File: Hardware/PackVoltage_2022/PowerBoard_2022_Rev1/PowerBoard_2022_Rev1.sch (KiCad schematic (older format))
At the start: 0 parts

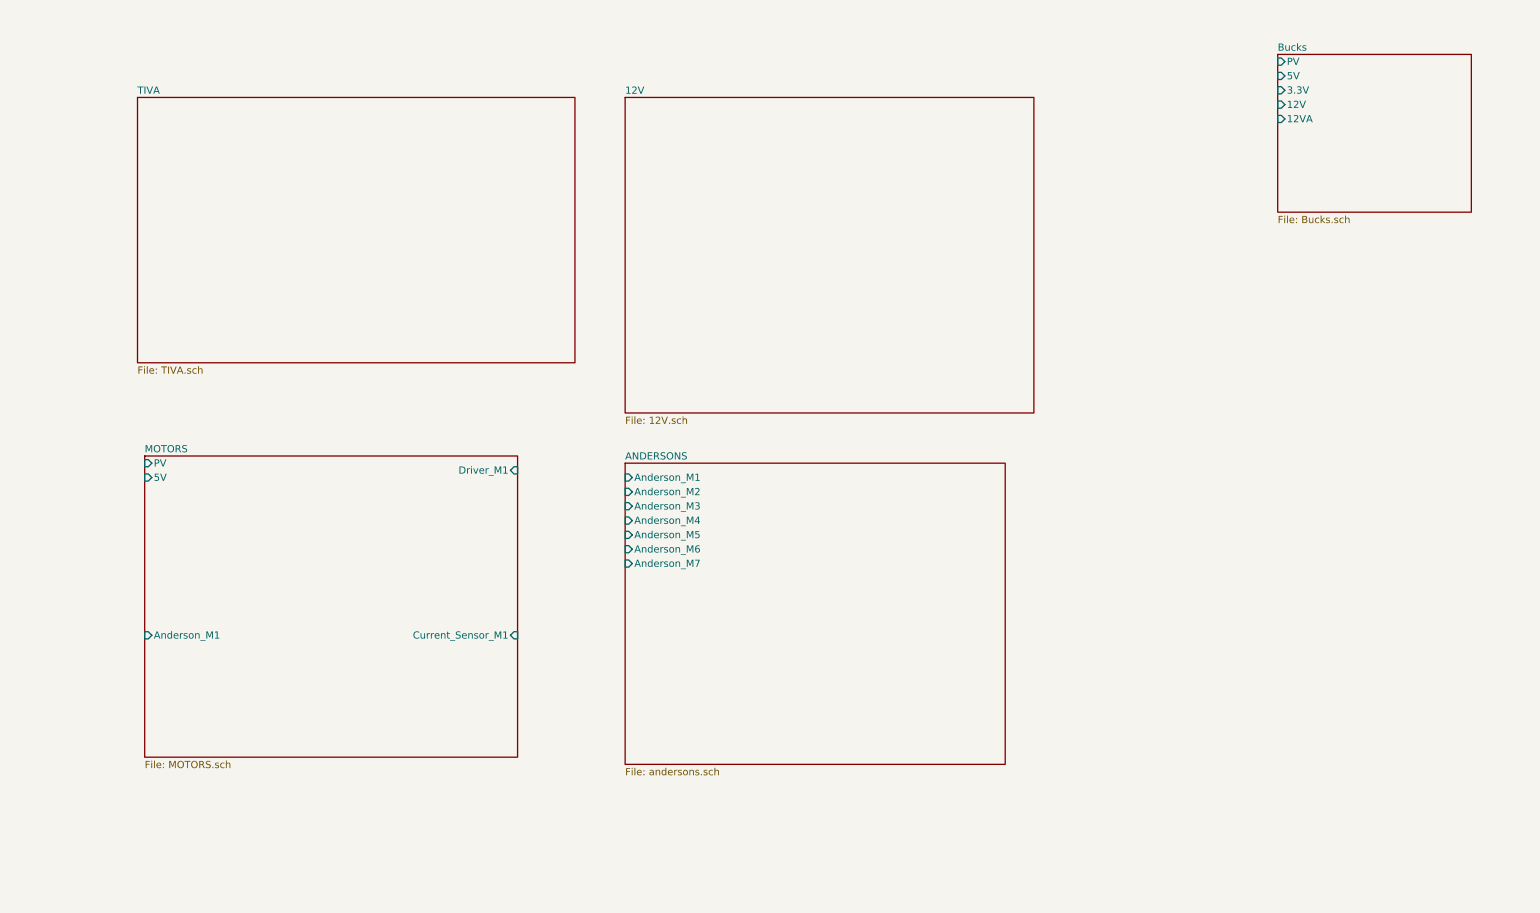
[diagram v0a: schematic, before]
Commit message: 12V stuff and hierarchical tags
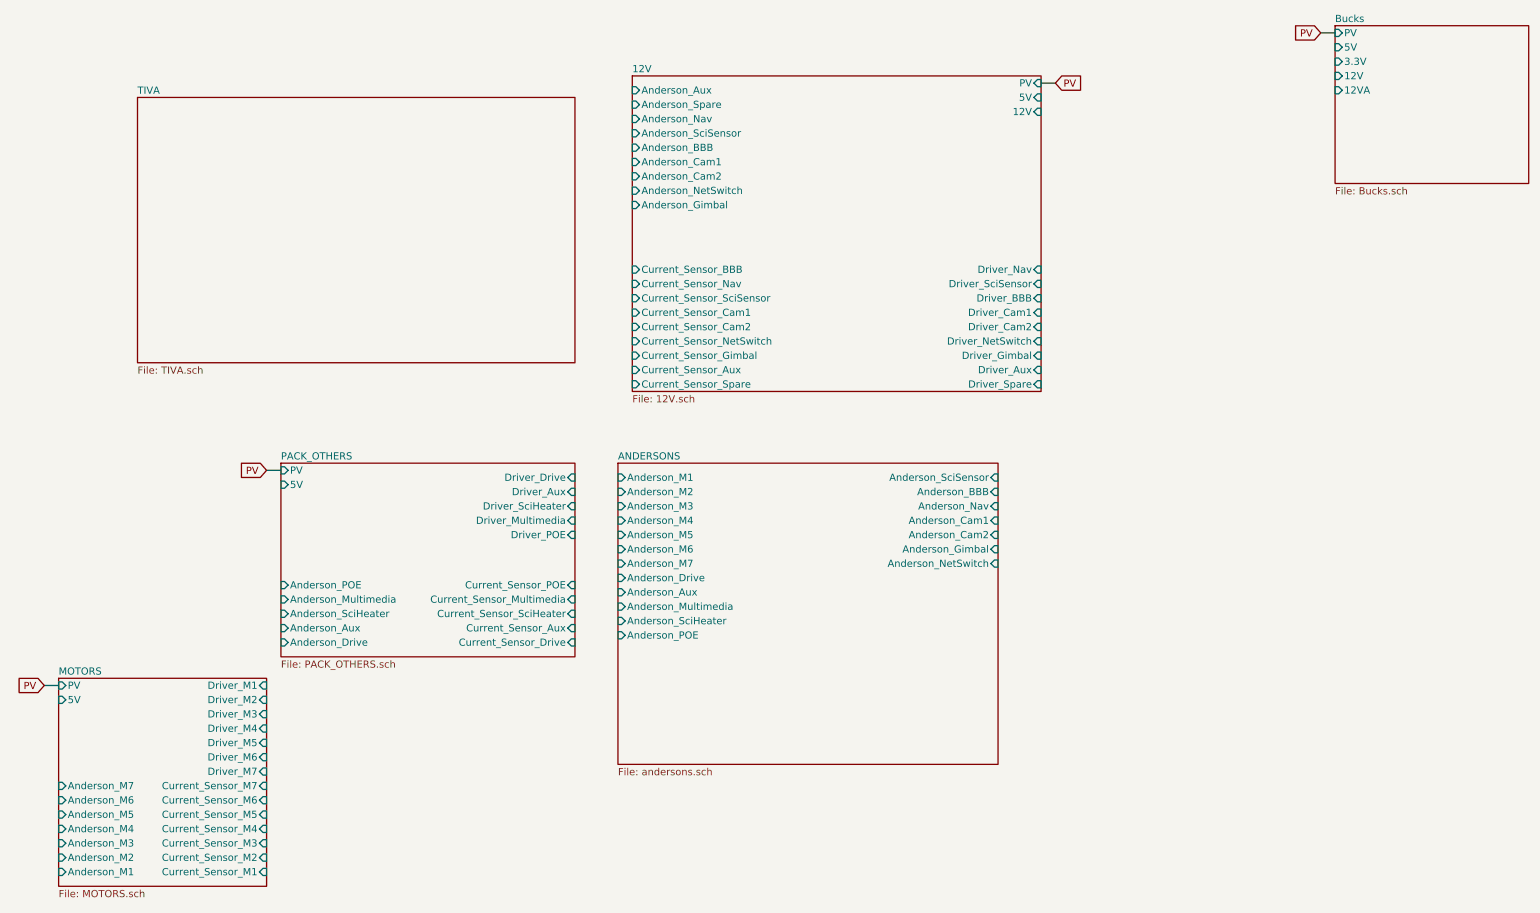
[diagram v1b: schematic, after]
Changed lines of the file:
@@
 $Descr A4 11693 8268
 encoding utf-8
-Sheet 1 8
+Sheet 1 10
 Title ""
 Date ""
@@
 $EndDescr
 $Sheet
-S 9350 850  1350 1100
+S 9750 650  1350 1100
 U 61563C60
 F0 "Bucks" 50
 F1 "Bucks.sch" 50
-F2 "PV" I L 9350 900 50
-F3 "5V" I L 9350 1000 50
-F4 "3.3V" I L 9350 1100 50
-F5 "12V" I L 9350 1200 50
-F6 "12VA" I L 9350 1300 50
+F2 "PV" I L 9750 700 50
+F3 "5V" I L 9750 800 50
+F4 "3.3V" I L 9750 900 50
+F5 "12V" I L 9750 1000 50
+F6 "12VA" I L 9750 1100 50
 $EndSheet
 $Sheet
@@
 $EndSheet
 $Sheet
-S 4800 3700 2650 2100
+S 4750 3700 2650 2100
 U 615E92DD
 F0 "ANDERSONS" 50
 F1 "andersons.sch" 50
-F2 "Anderson_M2" I L 4800 3900 50
-F3 "Anderson_M1" I L 4800 3800 50
-F4 "Anderson_M3" I L 4800 4000 50
-F5 "Anderson_M4" I L 4800 4100 50
-F6 "Anderson_M5" I L 4800 4200 50
-F7 "Anderson_M6" I L 4800 4300 50
-F8 "Anderson_M7" I L 4800 4400 50
+F2 "Anderson_M2" I L 4750 3900 50
+F3 "Anderson_M1" I L 4750 3800 50
+F4 "Anderson_M3" I L 4750 4000 50
+F5 "Anderson_M4" I L 4750 4100 50
+F6 "Anderson_M5" I L 4750 4200 50
+F7 "Anderson_M6" I L 4750 4300 50
+F8 "Anderson_M7" I L 4750 4400 50
+F9 "Anderson_Drive" I L 4750 4500 50
+F10 "Anderson_Aux" I L 4750 4600 50
+F11 "Anderson_Multimedia" I L 4750 4700 50
+F12 "Anderson_SciHeater" I L 4750 4800 50
+F13 "Anderson_POE" I L 4750 4900 50
+F14 "Anderson_SciSensor" I R 7400 3800 50
+F15 "Anderson_BBB" I R 7400 3900 50
+F16 "Anderson_Nav" I R 7400 4000 50
+F17 "Anderson_Cam1" I R 7400 4100 50
+F18 "Anderson_Cam2" I R 7400 4200 50
+F19 "Anderson_Gimbal" I R 7400 4300 50
+F20 "Anderson_NetSwitch" I R 7400 4400 50
 $EndSheet
 $Sheet
-S 1450 3650 2600 2100
+S 850  5200 1450 1450
 U 615D5992
 F0 "MOTORS" 50
 F1 "MOTORS.sch" 50
-F2 "PV" I L 1450 3700 50
-F3 "5V" I L 1450 3800 50
-F4 "Anderson_M1" I L 1450 4900 50
-F5 "Driver_M1" I R 4050 3750 50
-F6 "Current_Sensor_M1" I R 4050 4900 50
+F2 "PV" I L 850 5250 50
+F3 "5V" I L 850 5350 50
+F4 "Anderson_M1" I L 850 6550 50
+F5 "Driver_M1" I R 2300 5250 50
+F6 "Current_Sensor_M1" I R 2300 6550 50
+F7 "Anderson_M2" I L 850 6450 50
+F8 "Driver_M2" I R 2300 5350 50
+F9 "Current_Sensor_M2" I R 2300 6450 50
+F10 "Anderson_M3" I L 850 6350 50
+F11 "Driver_M3" I R 2300 5450 50
+F12 "Current_Sensor_M3" I R 2300 6350 50
+F13 "Anderson_M4" I L 850 6250 50
+F14 "Driver_M4" I R 2300 5550 50
+F15 "Current_Sensor_M4" I R 2300 6250 50
+F16 "Anderson_M5" I L 850 6150 50
+F17 "Driver_M5" I R 2300 5650 50
+F18 "Current_Sensor_M5" I R 2300 6150 50
+F19 "Anderson_M7" I L 850 5950 50
+F20 "Driver_M7" I R 2300 5850 50
+F21 "Current_Sensor_M7" I R 2300 5950 50
+F22 "Anderson_M6" I L 850 6050 50
+F23 "Driver_M6" I R 2300 5750 50
+F24 "Current_Sensor_M6" I R 2300 6050 50
 $EndSheet
 $Sheet
-S 4800 1150 2850 2200
+S 4850 1000 2850 2200
 U 615D7BA0
 F0 "12V" 50
 F1 "12V.sch" 50
+F2 "Anderson_Aux" I L 4850 1100 50
+F3 "PV" I R 7700 1050 50
+F4 "5V" I R 7700 1150 50
+F5 "Anderson_Spare" I L 4850 1200 50
+F6 "Anderson_Nav" I L 4850 1300 50
+F7 "Anderson_SciSensor" I L 4850 1400 50
+F8 "Anderson_BBB" I L 4850 1500 50
+F9 "Anderson_Cam1" I L 4850 1600 50
+F10 "Anderson_Cam2" I L 4850 1700 50
+F11 "Anderson_NetSwitch" I L 4850 1800 50
+F12 "Anderson_Gimbal" I L 4850 1900 50
+F13 "12V" I R 7700 1250 50
+F14 "Driver_Nav" I R 7700 2350 50
+F15 "Driver_SciSensor" I R 7700 2450 50
+F16 "Driver_BBB" I R 7700 2550 50
+F17 "Driver_Cam1" I R 7700 2650 50
+F18 "Driver_Cam2" I R 7700 2750 50
+F19 "Driver_NetSwitch" I R 7700 2850 50
+F20 "Driver_Gimbal" I R 7700 2950 50
+F21 "Driver_Aux" I R 7700 3050 50
+F22 "Driver_Spare" I R 7700 3150 50
+F23 "Current_Sensor_BBB" I L 4850 2350 50
+F24 "Current_Sensor_Nav" I L 4850 2450 50
+F25 "Current_Sensor_SciSensor" I L 4850 2550 50
+F26 "Current_Sensor_Cam1" I L 4850 2650 50
+F27 "Current_Sensor_Cam2" I L 4850 2750 50
+F28 "Current_Sensor_NetSwitch" I L 4850 2850 50
+F29 "Current_Sensor_Gimbal" I L 4850 2950 50
+F30 "Current_Sensor_Aux" I L 4850 3050 50
+F31 "Current_Sensor_Spare" I L 4850 3150 50
 $EndSheet
+$Sheet
+S 2400 3700 2050 1350
+U 61609A41
+F0 "PACK_OTHERS" 50
+F1 "PACK_OTHERS.sch" 50
+F2 "PV" I L 2400 3750 50
+F3 "5V" I L 2400 3850 50
+F4 "Anderson_Drive" I L 2400 4950 50
+F5 "Driver_Drive" I R 4450 3800 50
+F6 "Current_Sensor_Drive" I R 4450 4950 50
+F7 "Anderson_Aux" I L 2400 4850 50
+F8 "Driver_Aux" I R 4450 3900 50
+F9 "Current_Sensor_Aux" I R 4450 4850 50
+F10 "Anderson_SciHeater" I L 2400 4750 50
+F11 "Driver_SciHeater" I R 4450 4000 50
+F12 "Current_Sensor_SciHeater" I R 4450 4750 50
+F13 "Anderson_Multimedia" I L 2400 4650 50
+F14 "Driver_Multimedia" I R 4450 4100 50
+F15 "Current_Sensor_Multimedia" I R 4450 4650 50
+F16 "Anderson_POE" I L 2400 4550 50
+F17 "Driver_POE" I R 4450 4200 50
+F18 "Current_Sensor_POE" I R 4450 4550 50
+$EndSheet
+Text GLabel 9650 700  0    50   Input ~ 0
+PV
+Wire Wire Line
+	9650 700  9750 700
+Text GLabel 7800 1050 2    50   Input ~ 0
+PV
+Wire Wire Line
+	7800 1050 7700 1050
+Text GLabel 2300 3750 0    50   Input ~ 0
+PV
+Wire Wire Line
+	2300 3750 2400 3750
+Text GLabel 750  5250 0    50   Input ~ 0
+PV
+Wire Wire Line
+	750  5250 850  5250
 $EndSCHEMATC
